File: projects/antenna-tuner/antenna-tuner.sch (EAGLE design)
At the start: 74 parts, among them J1 Power Jack, T1 BC337, T2 BC337, T3 BC337, U1 DC-DC Converter, U2 K155ID1, U3 Arduino Pro Mini, U4 Pollin DCF1, U5 REG1117

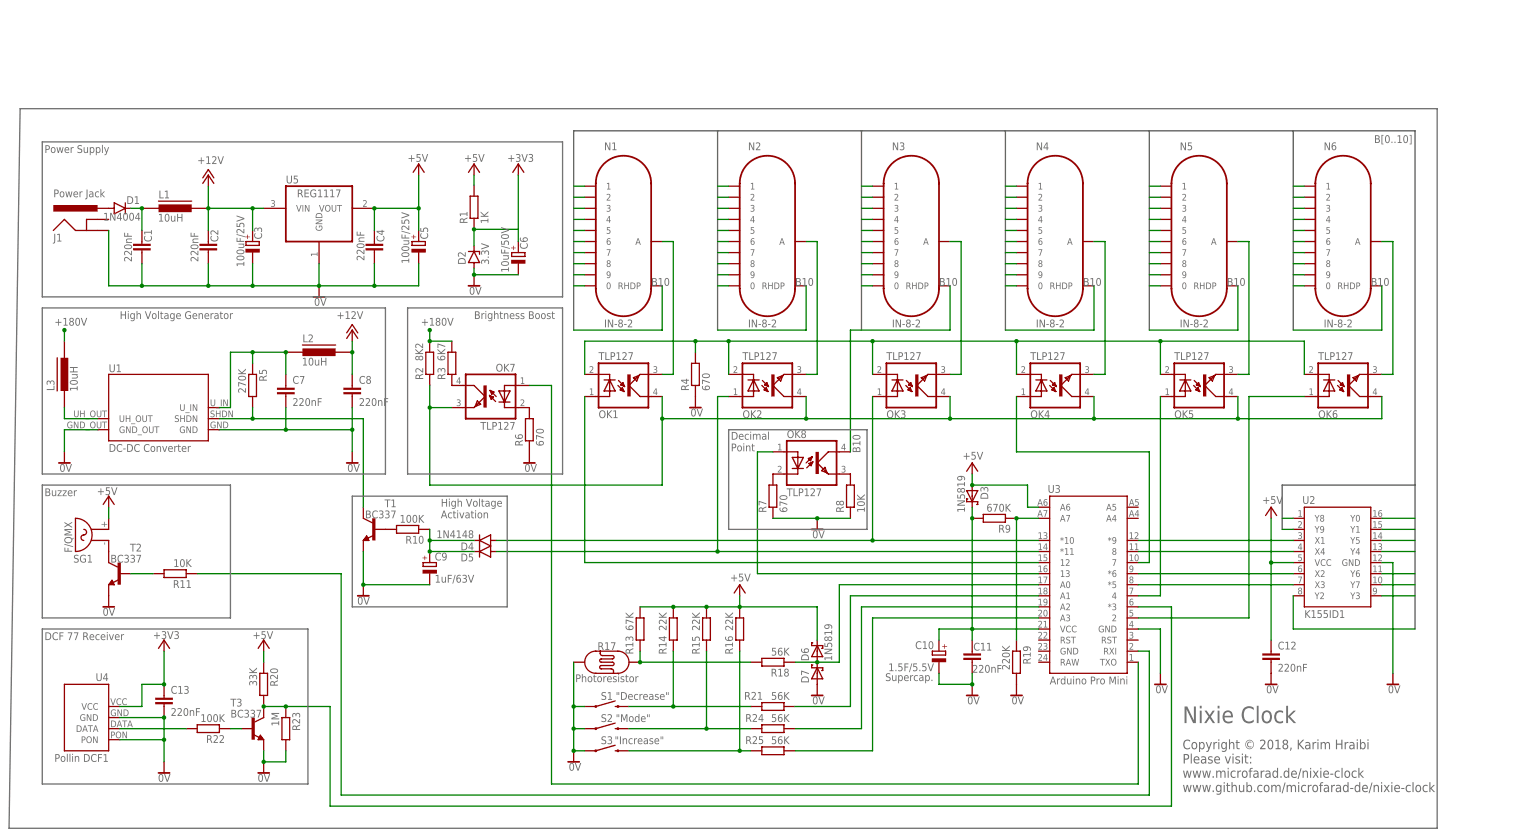
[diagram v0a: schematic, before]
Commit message: Created schematic for the antenna tuner
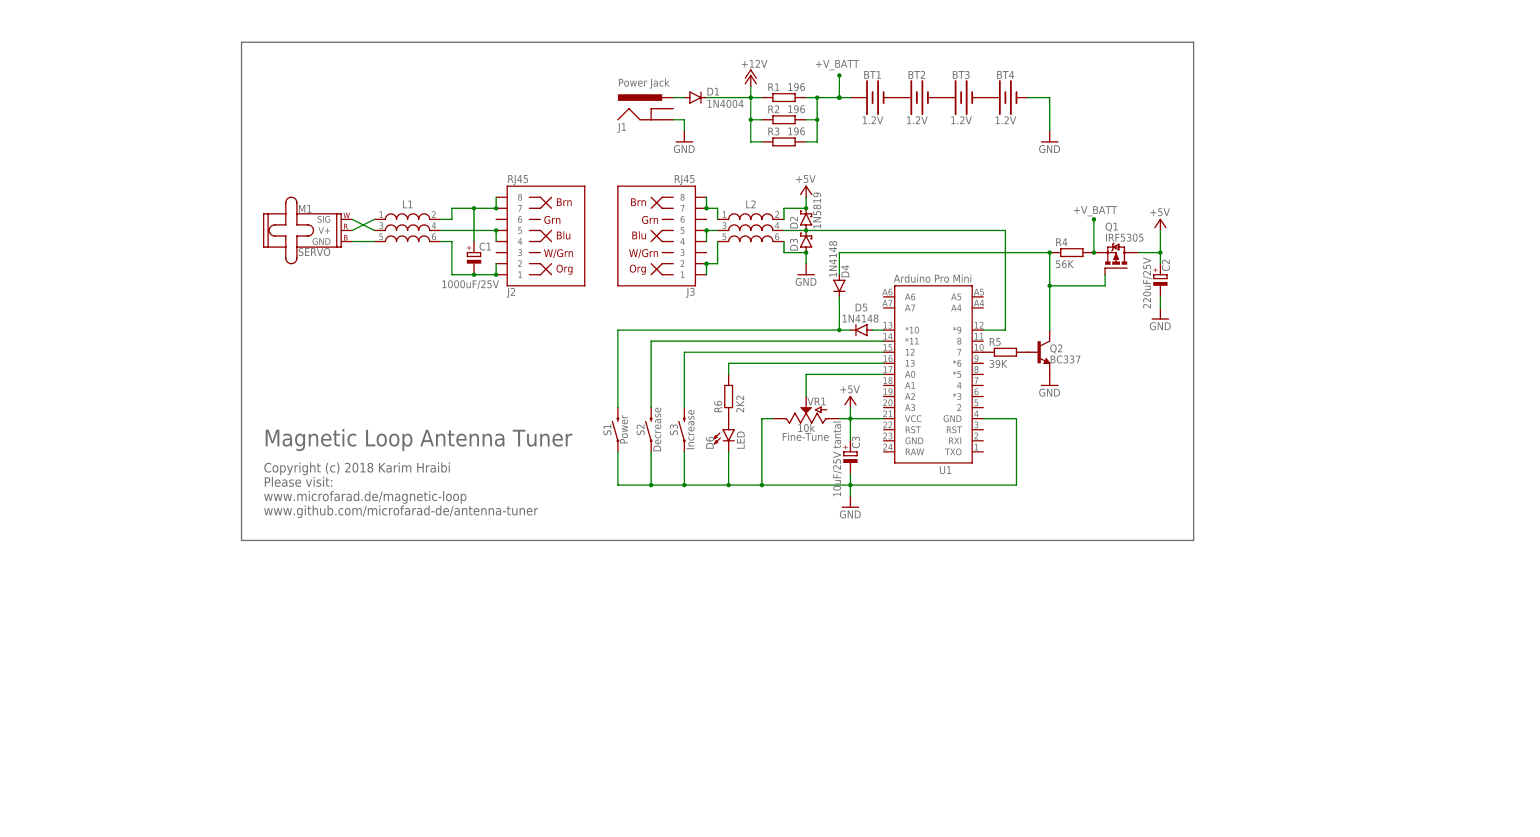
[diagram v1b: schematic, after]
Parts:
- removed C10: 1.5F/5.5V, karim:SUPERCAP/1.5F/5.5V
- removed C11, C12, C13, C4, C7, C8: 220nF, rcl:C-EU025-024X044
- removed C5: 100uF/25V, rcl:CPOL-EUE2.5-6
- removed C6: 10uF/50V, rcl:CPOL-EUE2-4
- removed C9: 1uF/63V, rcl:CPOL-EUE1.8-4
- removed D7: 1N5819, diode:1N5819-B
- removed L3: 10uH, microfarad-de:CHOKE/9.5MM
- removed N1, N2, N3, N4, N5, N6: IN-8-2, russian-nixies:IN-8-2
- removed OK1, OK2, OK3, OK4, OK5, OK6, OK7, OK8: TLP127, karim:TLP127
- removed R10, R22: 100K, rcl:R-EU_0207/7
- removed R11, R8: 10K, rcl:R-EU_0207/7
- removed R13: 67K, rcl:R-EU_0207/7
- removed R14, R15, R16: 22K, rcl:R-EU_0207/7
- removed R17: Photoresistor, SparkFun-Sensors:PHOTOCELLPTH
- removed R18, R21, R24, R25: 56K, rcl:R-EU_0207/7
- removed R19: 220K, rcl:R-EU_0207/7
- removed R20: 33K, rcl:R-EU_0207/7
- removed R23: 1M, rcl:R-EU_0207/7
- removed R7: 670, rcl:R-EU_0207/7
- removed R9: 670K, rcl:R-EU_0207/7
- removed SG1: F/QMX, buzzer:F/QMX
- removed T1, T2, T3: BC337, transistor:BC337
- removed U2: K155ID1, karim:K155ID1
- removed U3: Arduino Pro Mini, karim:ARDUINO_PRO_MINI_TS
- removed U4: Pollin DCF1, karim:DCF1
- removed U5: REG1117, burr-brown:REG1117
- added BT1, BT2, BT3, BT4: 1.2V, SparkFun-Batteries:BATTERY-AA
- added J2, J3: RJ45, SparkFun-Connectors:RJ45-8
- added M1: SERVO, SparkFun-Electromechanical:SERVO
- added Q1: IRF5305, microfarad-de:IRF5305
- added Q2: BC337, transistor-npn:BC337
- added VR1: 10k, SparkFun-Resistors:POTENTIOMETER-PTH-9MM-1/20W-20%
- C1: value 220nF -> 1000uF/25V; device rcl:C-EU025-024X044 -> rcl:CPOL-EUE5-10.5
- C2: value 220nF -> 220uF/25V; device rcl:C-EU025-024X044 -> rcl:CPOL-EUE2.5-6
- C3: value 100uF/25V -> 10uF/25V tantal
- D2: value 3.3V -> 1N5819; device diode:ZENER-DIODEZD-5 -> diode:1N5819-B
- D6: value 1N5819 -> LED; device diode:1N5819-B -> SparkFun-LED:LED5MM
- J1: device SparkFun-Connectors:POWER_JACKSLT -> SparkFun-Connectors:POWER_JACKPTH_BREAD
- L1, L2: value 10uH -> (none); device microfarad-de:CHOKE/9.5MM -> Wurth_Elektronik_Passive_rev18f:WE-MLS-3WAY_74273001
- R1: value 1K -> 196
- R2: value 8K2 -> 196
- R3: value 6K7 -> 196
- R4: value 670 -> 56K
- R5: value 270K -> 39K
- R6: value 670 -> 2K2
- S1: value "Decrease" -> Power
- S2: value "Mode" -> Decrease
- S3: value "Increase" -> Increase
- U1: value DC-DC Converter -> Arduino Pro Mini; device karim:CHINA_HV_DC_DC -> microfarad-de:ARDUINO_PRO_MINI_TS
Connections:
- removed net +180V: L3.2, R2.2, R3.2
- removed net +3V3: C13.1, C6.+, D2.C, R1.1, U4.VCC
- removed net 0V: C1.2, C10.-, C11.2, C12.2, C13.2, C2.2, C3.-, C4.2, C5.-, C6.-, C7.2, C8.2, C9.-, D2.A, D7.A, J1.GND, R17.P$1, R19.2, R23.2, R4.1, R6.1, R7.1, R8.1, S1.1, S2.1, S3.1, T1.E, T2.E, T3.E, U1.GND, U1.GND_OUT, U2.GND, U3.GND, U4.GND, U4.PON, U5.GND
- removed net 180VRAW: L3.1, U1.UH_OUT
- removed net B0: N1.0, N2.0, N3.0, N4.0, N5.0, N6.0, U2.Y0
- removed net B1: N1.1, N2.1, N3.1, N4.1, N5.1, N6.1, U2.Y1
- removed net B10: N1.RHDP, N2.RHDP, N3.RHDP, N4.RHDP, N5.RHDP, N6.RHDP, OK8.COL
- removed net B2: N1.2, N2.2, N3.2, N4.2, N5.2, N6.2, U2.Y2
- removed net B3: N1.3, N2.3, N3.3, N4.3, N5.3, N6.3, U2.Y3
- removed net B4: N1.4, N2.4, N3.4, N4.4, N5.4, N6.4, U2.Y4
- removed net B5: N1.5, N2.5, N3.5, N4.5, N5.5, N6.5, U2.Y5
- removed net B6: N1.6, N2.6, N3.6, N4.6, N5.6, N6.6, U2.Y6
- removed net B7: N1.7, N2.7, N3.7, N4.7, N5.7, N6.7, U2.Y7
- removed net B8: N1.8, N2.8, N3.8, N4.8, N5.8, N6.8, U2.Y8
- removed net B9: N1.9, N2.9, N3.9, N4.9, N5.9, N6.9, U2.Y9
- removed net N$1 (its old number): N6.A, OK6.EMIT
- removed net N$24: OK8.A, U3.13
- removed net N$26: C1.1, D1.C, L1.1
- removed net N$27: R20.2, R23.1, T3.C, U3.*3
- removed net N$28: R11.2, T2.B
- removed net N$29: R22.1, T3.B
- removed net N$30: R22.2, U4.DATA
- removed net N$31: SG1.1, T2.C
- removed net N$32: R11.1, U3.RXI
- removed net N$33: C10.+, C11.1, D3.C, R9.2, U3.VCC
- removed net N$34: R19.1, R9.1, U3.A7
- removed net N$35: D6.A, D7.C, R18.1, U3.A0
- removed net N$36: R13.2, R17.P$2, R18.2
- removed net N$37: R14.2, R21.2, S1.2
- removed net N$38: R15.2, R24.2, S2.2
- removed net N$39: R16.2, R25.2, S3.2
- removed net N$40: R21.1, U3.A1
- removed net N$41: R24.1, U3.A2
- removed net N$42: R25.1, U3.A3
- removed net X1: U2.X1, U3.*9
- removed net X2: U2.X2, U3.*6
- removed net X3: U2.X3, U3.*5
- removed net X4: U2.X4, U3.8
- new net +V_BATT: BT1.+, Q1.S$1, R1.2, R2.2, R3.2, R4.2
- new net GND: BT4.-, C2.-, C3.-, D3.A, D6.C, J1.GND, L2.6, Q2.E, S1.1, S2.1, S3.1, U1.GND, VR1.E
- net +12V: now also D1.C, R1.1, R2.1, R3.1; no longer C2.1, C3.+, C8.1, L1.2, L2.2, U5.VIN
- net +5V: now also C2.+, C3.+, D2.C, L2.2, Q1.D$1, U1.VCC, VR1.A; no longer C12.1, C4.1, C5.+, D3.A, D6.C, R1.2, R13.1, R14.1, R15.1, R16.1, R20.1, SG1.2, U2.VCC, U3.A6, U5.VOUT
- net N$10: now also S3.2, U1.12; no longer OK5.A, U3.4
- net N$11: now also S2.2, U1.*11; no longer OK4.A, U3.7
- net N$12: now also D5.A, U1.*10; no longer D4.A, OK3.A, U3.*10
- net N$13: now also D4.C, D5.C, S1.2; no longer D5.A, OK2.A, U3.*11
- net N$14: now also D2.A, D3.C, L2.4, U1.*9; no longer OK1.A, U3.12
- net N$15: now also J3.1, J3.2, L2.5; no longer C7.1, L2.1, R5.1, U1.U_IN
- net N$16: now also J3.7, J3.8, L2.1; no longer R10.2, T1.B
- net N$17: now also J3.4, J3.5, L2.3; no longer C9.+, D4.C, D5.C, R10.1
- net N$18: now also C1.+, J2.7, J2.8, L1.2; no longer R5.2, T1.C, U1.SHDN
- net N$19: now also J2.4, J2.5, L1.4; no longer OK1.C, OK2.C, OK3.C, OK4.C, OK5.C, OK6.C, R4.2
- net N$2: now also BT1.-, BT2.+; no longer N5.A, OK5.EMIT
- net N$20: now also C1.-, J2.1, J2.2, L1.6; no longer OK7.C, R6.2
- net N$21: now also L1.1, M1.V+; no longer OK7.A, U3.TXO
- net N$22: now also L1.5, M1.GND; no longer OK8.EMIT, R8.2
- net N$23: now also L1.3, M1.SIG; no longer OK8.C, R7.2
- net N$3: now also BT3.-, BT4.+; no longer N4.A, OK4.EMIT
- net N$4: now also BT2.-, BT3.+; no longer N3.A, OK3.EMIT
- net N$5: now also U1.A0, VR1.S; no longer N2.A, OK2.EMIT
- net N$6: now also Q2.B, R5.1, R5.2, U1.7; no longer N1.A, OK1.EMIT
- net N$7: now also D6.A, R6.1; no longer OK1.COL, OK2.COL, OK3.COL, OK4.COL, OK5.COL, OK6.COL, OK7.EMIT, R2.1
- net N$8: now also D4.A, Q1.G$1, Q2.C, R4.1; no longer OK7.COL, R3.1
- net N$9: now also R6.2, U1.13; no longer OK6.A, U3.2
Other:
- note added: "Copyright (c) 2018 Karim Hraibi Please visit: www.microfarad.de/magnetic-loop www.github.com/microfarad-de/antenna-tuner"
- note added: "Fine-Tune"
- note added: "Magnetic Loop Antenna Tuner"
- note removed: "Brightness Boost"
- note removed: "Buzzer"
- note removed: "Copyright © 2018, Karim Hraibi Please visit: www.microfarad.de/nixie-clock www.github.com/microfarad-de/nixie-clock"
- note removed: "DCF 77 Receiver"
- note removed: "Decimal Point"
- note removed: "High Voltage Activation"
- note removed: "High Voltage Generator"
- note removed: "Nixie Clock"
- note removed: "Power Supply"
- note removed: "Supercap."
- moved on the sheet: C3, D1, D4, D5, D6, J1, R1, R2, R3, R4, R5, R6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

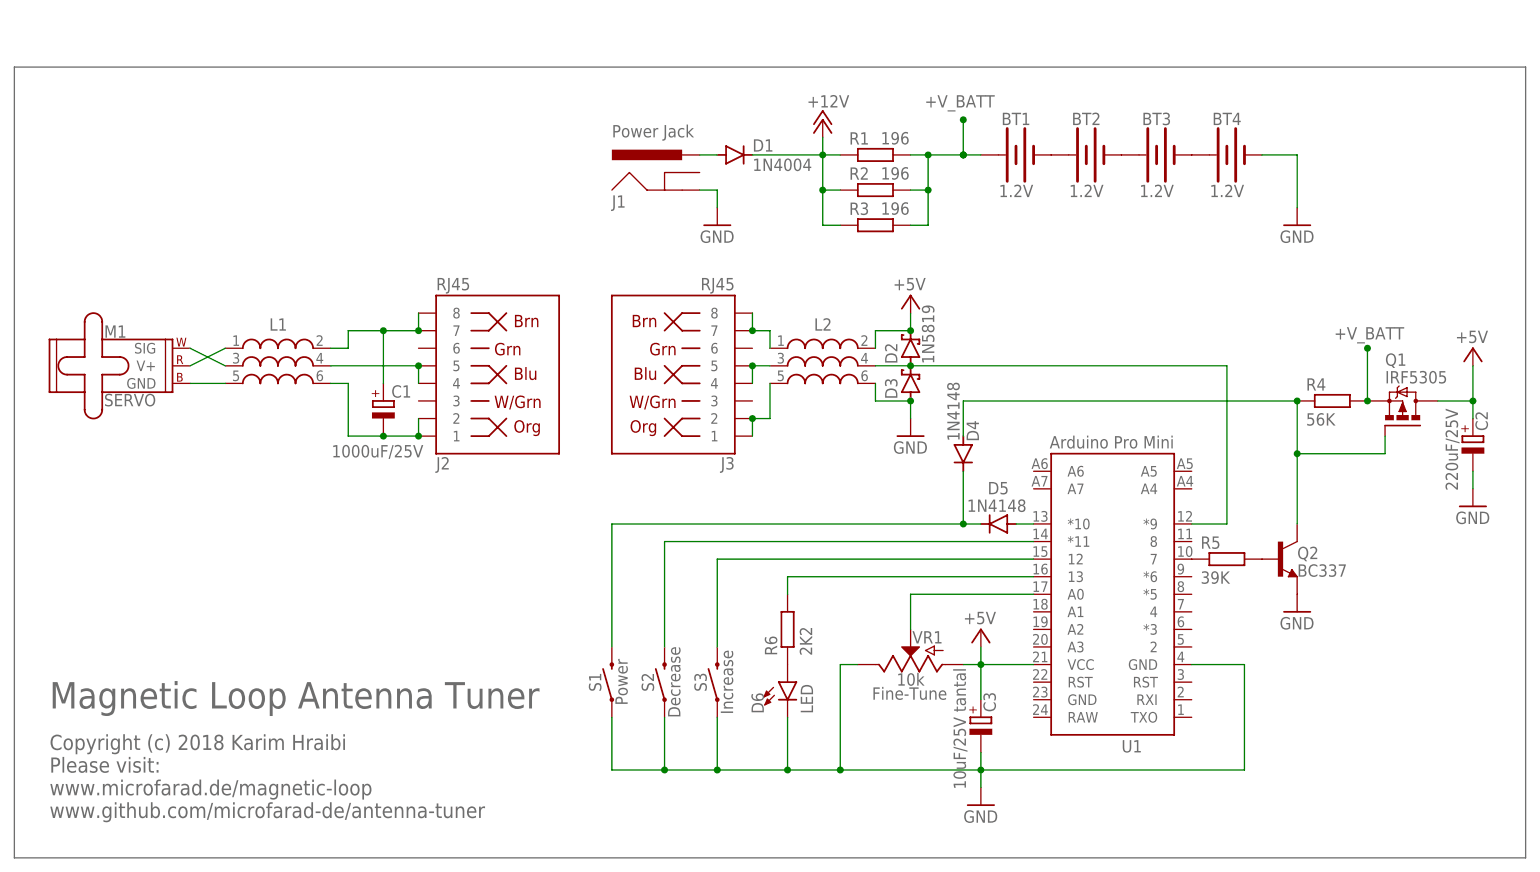
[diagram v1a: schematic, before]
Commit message: Update antenna-tuner.sch
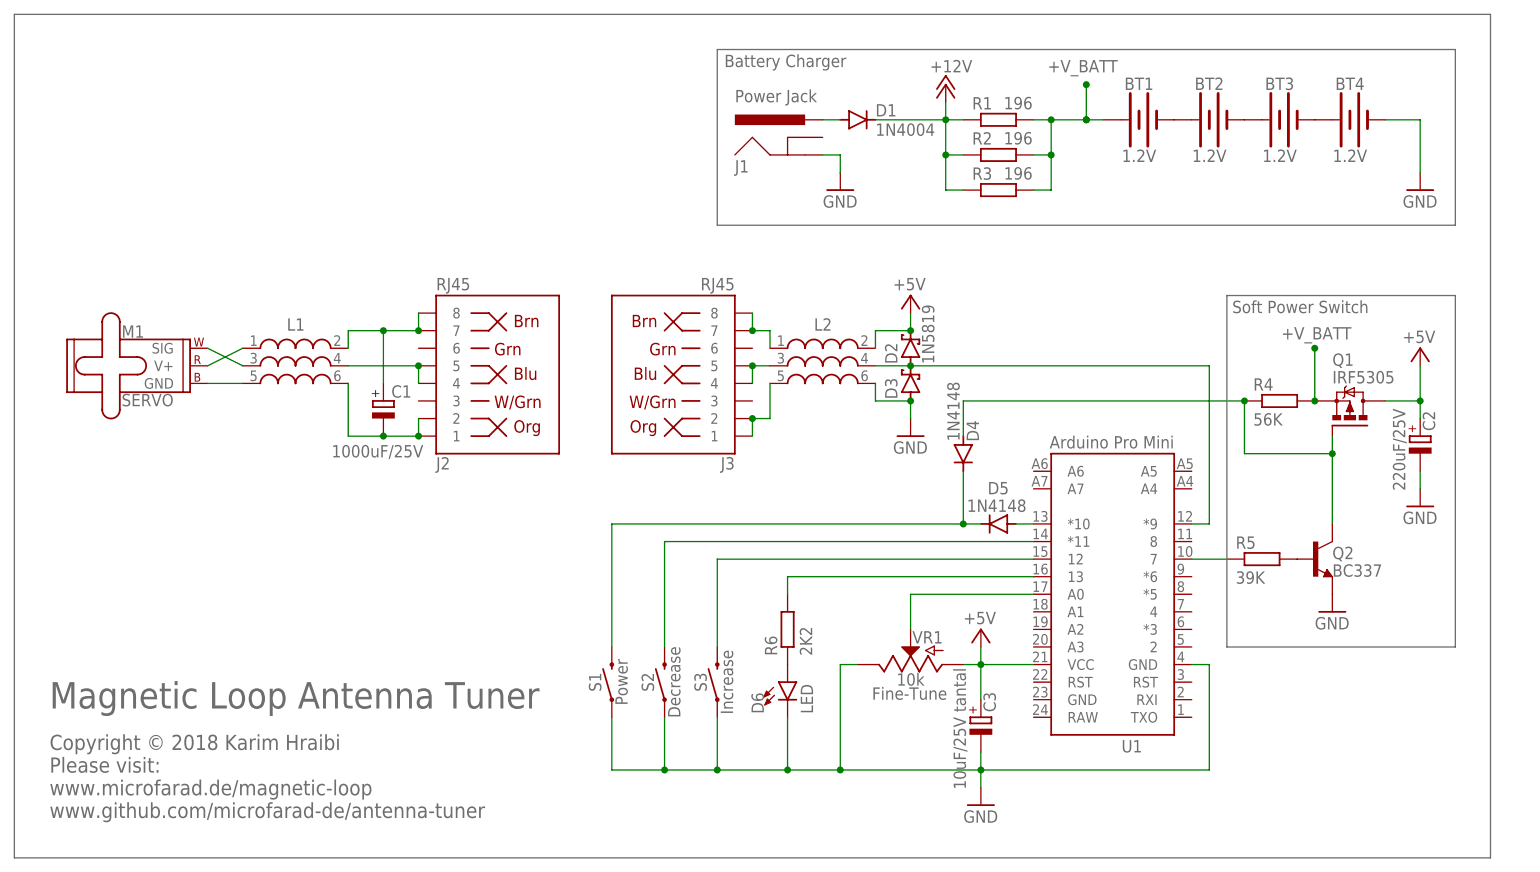
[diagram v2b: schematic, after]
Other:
- note added: "Battery Charger"
- note added: "Copyright © 2018 Karim Hraibi Please visit: www.microfarad.de/magnetic-loop www.github.com/microfarad-de/antenna-tuner"
- note added: "Soft Power Switch"
- note removed: "Copyright (c) 2018 Karim Hraibi Please visit: www.microfarad.de/magnetic-loop www.github.com/microfarad-de/antenna-tuner"
- moved on the sheet: BT1, BT2, BT3, BT4, C2, D1, J1, L1, M1, Q1, Q2, R1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
